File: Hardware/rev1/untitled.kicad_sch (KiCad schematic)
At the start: 15 parts, among them J3 Screw_Terminal_01x02, SW1 SW_Push, U2 HT75xx-1-SOT89

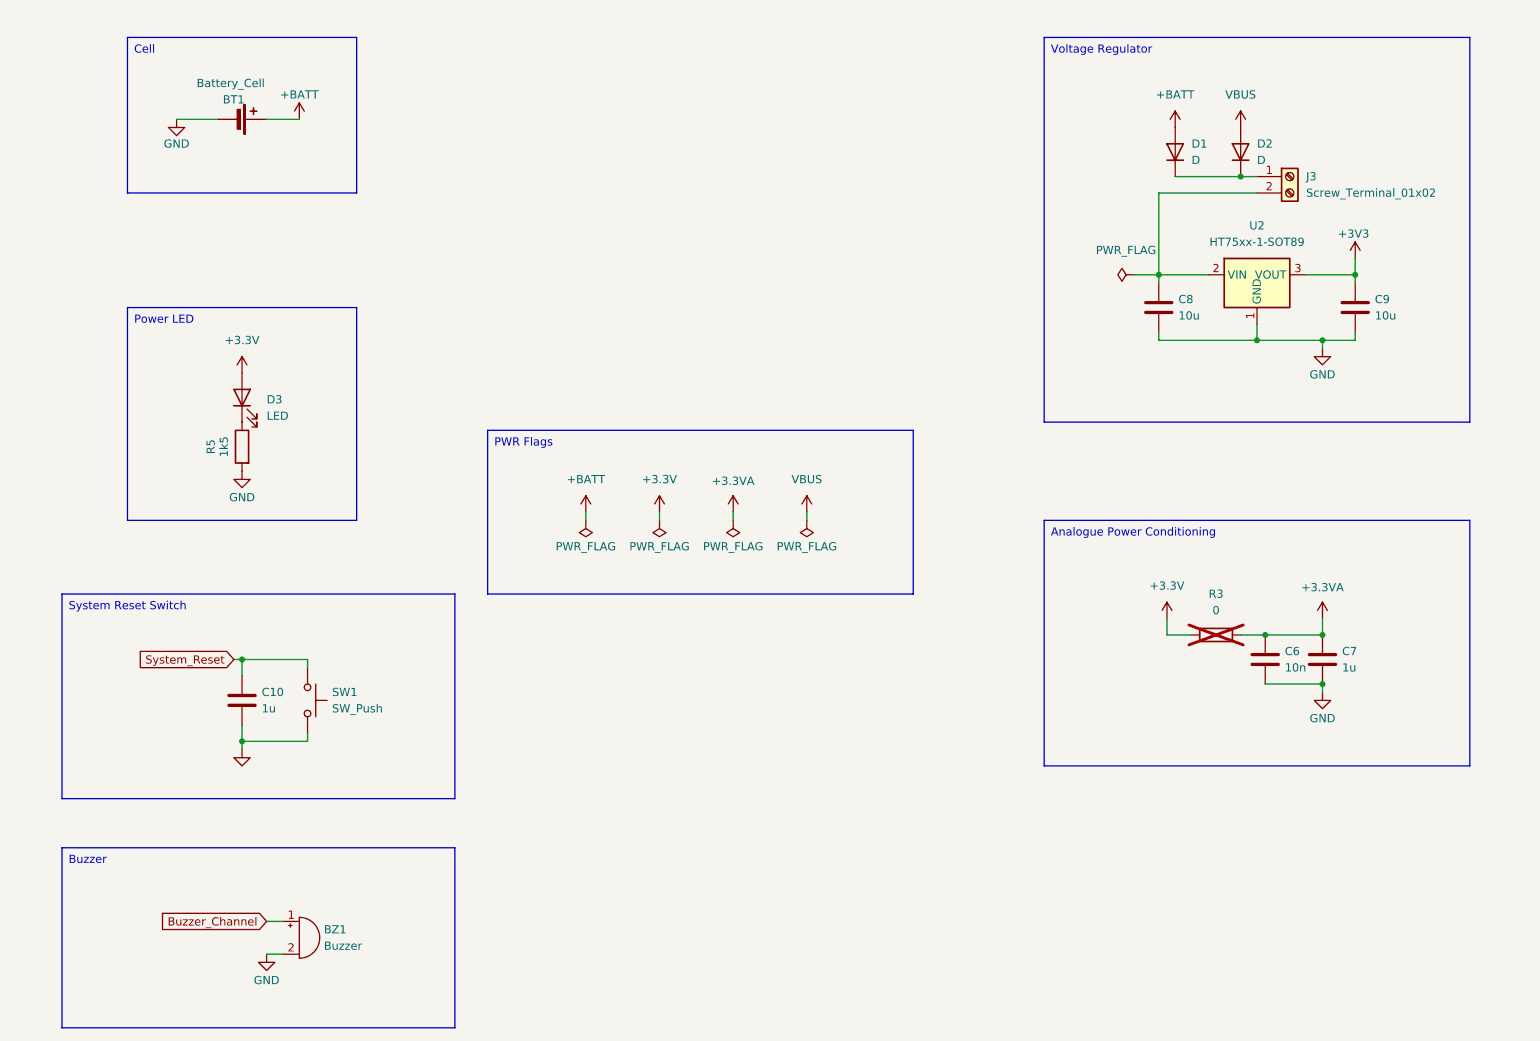
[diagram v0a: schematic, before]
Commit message: h
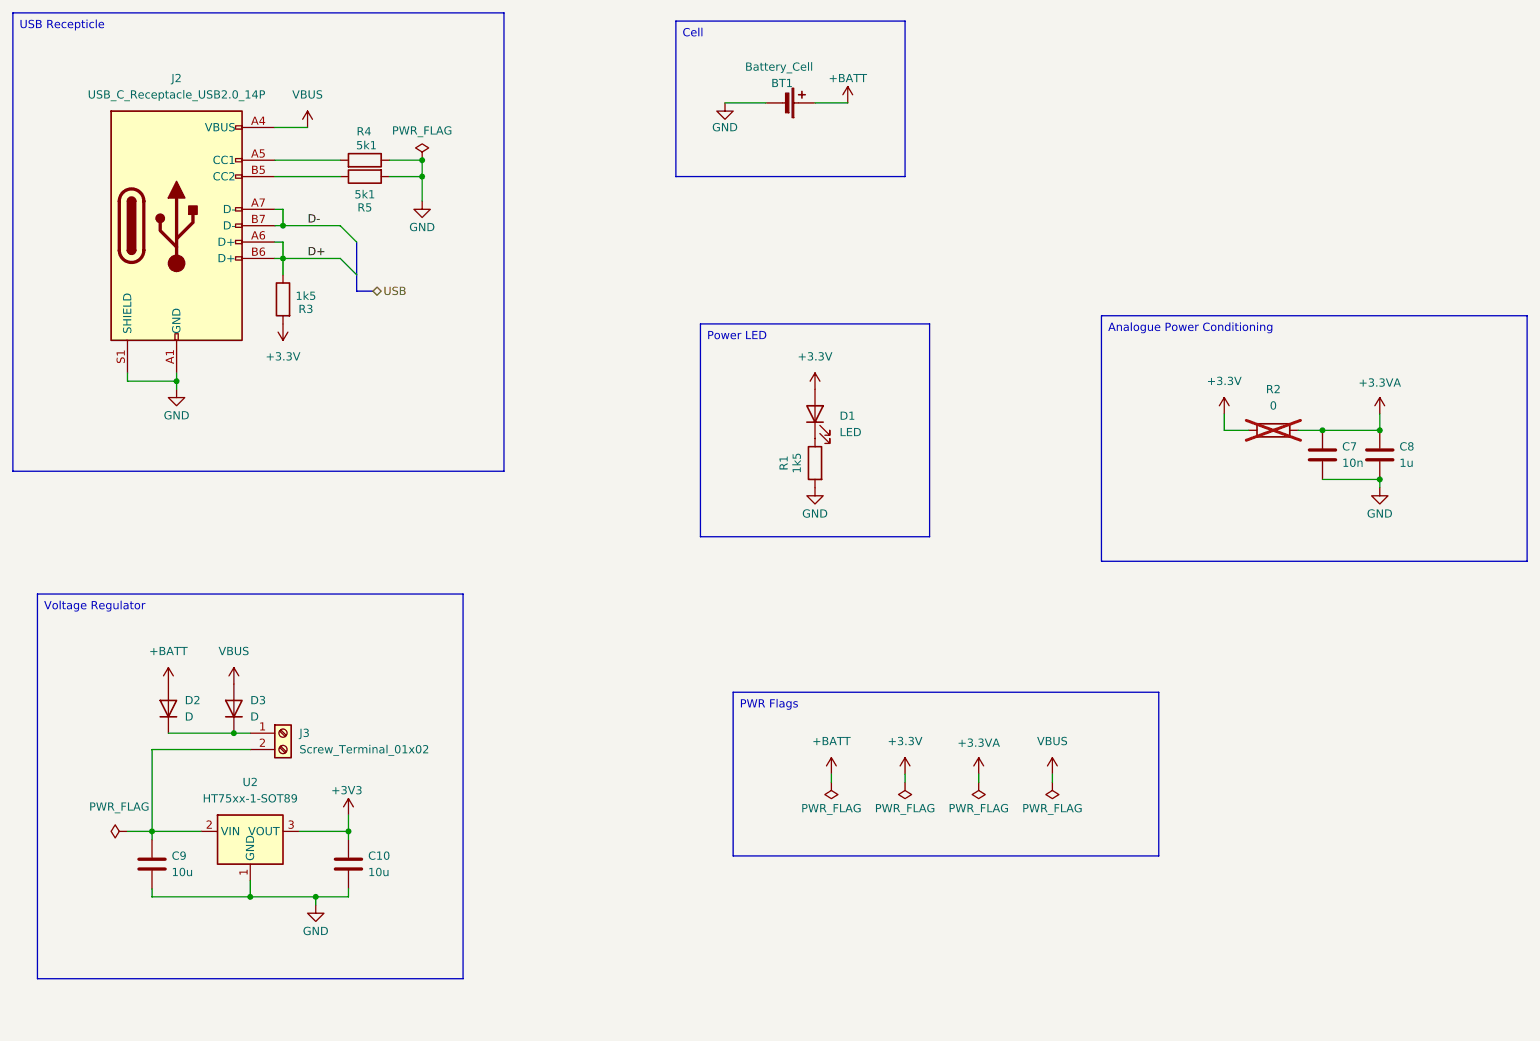
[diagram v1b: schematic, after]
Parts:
- removed BZ1: Buzzer, symbol Device:Buzzer
- removed C6: 10n, symbol Device:C
- removed D1: D, symbol Device:D
- removed D3: LED, symbol Device:LED
- removed SW1: SW_Push, symbol Switch:SW_Push
- added D1: LED, symbol Device:LED
- added D3: D, symbol Device:D
- added J2: USB_C_Receptacle_USB2.0_14P, symbol Connector:USB_C_Receptacle_USB2.0_14P
- added R1: 1k5, Resistor_SMD:R_0402_1005Metric, symbol Device:R
- added R2: 0, symbol Device:R
- added R4: 5k1, Resistor_SMD:R_0402_1005Metric, symbol Device:R
- C10: value 1u -> 10u
- C7: value 1u -> 10n
- C8: value 10u -> 1u
- R3: value 0 -> 1k5; footprint (none) -> Resistor_SMD:R_0402_1005Metric; now fitted
- R5: value 1k5 -> 5k1
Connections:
- net System_Reset is gone; now on net +3V3: C10.1
- net +3.3V: now also R3.2, D1.2 (A), R2.1; no longer R3.1
- net +3.3VA: now also C8.1, R2.2; no longer R3.2
- net +3V3: no longer C9.1
- net +BATT: now also D2.2 (A)
- net GND: now also J2.A1 (GND), J2.A12 (GND), J2.B1 (GND), J2.B12 (GND), J2.S1 (SHIELD), R1.2, R4.1
- net VBUS: now also D3.2 (A), J2.A4 (VBUS), J2.A9 (VBUS), J2.B4 (VBUS), J2.B9 (VBUS); no longer D2.2 (A)
- net at R5.1: now also J2.B5 (CC2)
- net at J3.2 (Pin_2), U2.2 (VIN): now also C9.1; no longer C8.1
- net at D2.1 (K), J3.1 (Pin_1): now also D3.1 (K)
- new net: D1.1 (K), R1.1
- new net: J2.A5 (CC1), R4.2
- new net D+: J2.A6 (D+), J2.B6 (D+), R3.1
- new net D-: J2.A7 (D-), J2.B7 (D-)
